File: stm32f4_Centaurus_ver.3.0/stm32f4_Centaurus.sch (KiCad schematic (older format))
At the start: 226 parts, among them IC1 PIC24FJ64GB004, J1 SERIAL1, J2 EXTERNAL_~RST, P1 PICKit3, P10 XA2_12V, P11 CAN0, P12 CAN1, P13 CAN0, P14 CAN1, P15 SERIAL2, P16 SERIAL0, P17 XA2_5V, P18 SWD, P2 SERIAL5_SBDBT, P23 A/D, P24 PWM, P25 A/D_batt, P26 PWM_batt, P27 EMERGENCY_CHECK, P28 I/O_5V, P29 I/O_Variable, P3 ENC0, P30 I/O_5V_batt, P31 I/O_Variable, P4 ENC2, P5 SPI0, P6 ENC3, P7 ENC1, P8 SERIAL4, P9 SERIAL3, Q1 FET_P, Q2 FET_P, Q3 FET_P, Q4 NPN, Q5 NPN, Q6 FET_P, Q7 FET_N, Q8 FET_N, SW1 Main_POWER, SW2 SW1, SW3 SW0, SW4 SW2, SW5 SW3, U1 STM32F407VG, U10 LOGO, U11 CPC1106N, U13 LOGO, U2 AZ1086H, U3 MCP2221A, U4 BD9G101G, U5 MAX3051, U6 MAX3051, U7 AQM1602_BL, U8 OSTBABS4C2B, U9 LOGO, X1 8MHz

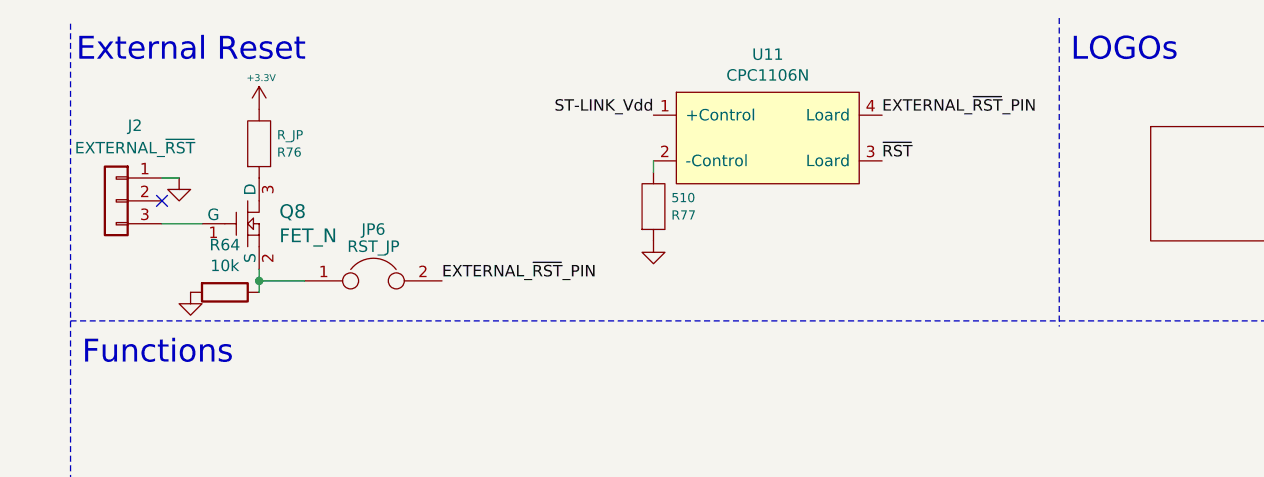
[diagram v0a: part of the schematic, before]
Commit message: 卍配　置　完　了卍
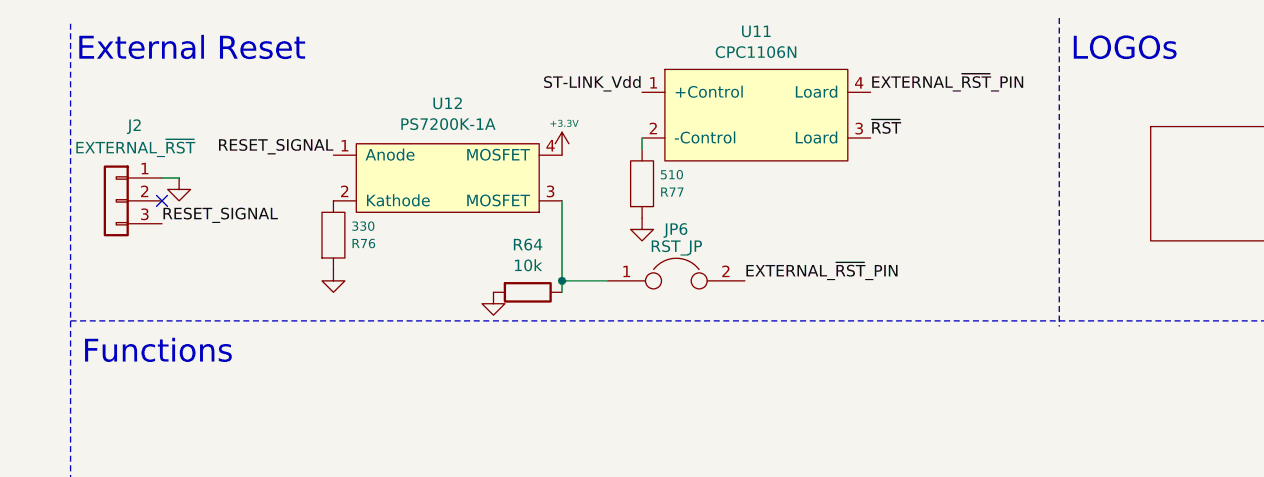
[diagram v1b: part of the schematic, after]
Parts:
- removed Q8: FET_N, Mizz_lib:SOT-23, symbol stm32f4_Centaurus-rescue:MOSFET_N_123-Hori_lib
- added U12: PS7200K-1A, Package_SO:SOP-4_3.8x4.1mm_P2.54mm, symbol Miz:PS7200K-1A
- R76: value R_JP -> 330
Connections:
- net +3V3: now also U12.4 (MOSFET); no longer R76.2
- net GND: now also R76.1
- net RESET_SIGNAL: now reaches J2.3 (Pin_3)
- net RESET_SIGNAL: now also U12.1 (Anode)
- net at JP6.1, R64.1: now also U12.3 (MOSFET)
- new net: R76.2, U12.2 (Kathode)
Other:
- moved on the sheet: JP6, R64, R77, U11
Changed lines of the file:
@@
 L stm32f4_Centaurus-rescue:GND-power #PWR0124
 U 1 1 5E845FAB
-P 17325 1425
-F 0 "#PWR0124" H 17325 1425 30  0001 C CNN
-F 1 "GND" H 17325 1355 30  0001 C CNN
-F 2 "" H 17325 1425 60  0000 C CNN
-F 3 "" H 17325 1425 60  0000 C CNN
-	1    17325 1425
+P 17275 1325
+F 0 "#PWR0124" H 17275 1325 30  0001 C CNN
+F 1 "GND" H 17275 1255 30  0001 C CNN
+F 2 "" H 17275 1325 60  0000 C CNN
+F 3 "" H 17275 1325 60  0000 C CNN
+	1    17275 1325
 	1    0    0    -1
 $EndComp
@@
 Text Label 2225 6825 0    50   ~ 0
 ~RST
-Text Label 18325 1075 0    50   ~ 0
+Text Label 18275 975  0    50   ~ 0
 ~RST
 $Comp
@@
 	1975 5900 2000 5900
 Connection ~ 1975 5900
-Text Label 17325 875  2    50   ~ 0
+Text Label 17275 775  2    50   ~ 0
 ST-LINK_Vdd
 $Comp
 L Miz:CPC1106N U11
 U 1 1 5E762683
-P 17825 975
-F 0 "U11" H 17825 1340 50  0000 C CNN
-F 1 "CPC1106N" H 17825 1249 50  0000 C CNN
-F 2 "Package_SO:SOP-4_3.8x4.1mm_P2.54mm" H 17825 1225 50  0001 C CNN
-F 3 "" H 17825 1225 50  0001 C CNN
-	1    17825 975
+P 17775 875
+F 0 "U11" H 17775 1240 50  0000 C CNN
+F 1 "CPC1106N" H 17775 1149 50  0000 C CNN
+F 2 "Package_SO:SOP-4_3.8x4.1mm_P2.54mm" H 17775 1125 50  0001 C CNN
+F 3 "" H 17775 1125 50  0001 C CNN
+	1    17775 875
 	1    0    0    -1
 $EndComp
@@
 L stm32f4_Centaurus-rescue:R-device R77
 U 1 1 5E7A7A85
-P 17325 1275
-F 0 "R77" H 17403 1313 40  0000 L CNN
-F 1 "510" H 17403 1237 40  0000 L CNN
-F 2 "Mizz_lib:1608_WP" V 17255 1275 30  0001 C CNN
-F 3 "" H 17325 1275 30  0000 C CNN
-	1    17325 1275
+P 17275 1175
+F 0 "R77" H 17353 1213 40  0000 L CNN
+F 1 "510" H 17353 1137 40  0000 L CNN
+F 2 "Mizz_lib:1608_WP" V 17205 1175 30  0001 C CNN
+F 3 "" H 17275 1175 30  0000 C CNN
+	1    17275 1175
 	1    0    0    1
 $EndComp
 Wire Wire Line
-	17325 1075 17325 1125
+	17275 975  17275 1025
 $Comp
 L stm32f4_Centaurus-rescue:+3.3V-power #PWR0139
 U 1 1 5E766875
-P 15600 850
-F 0 "#PWR0139" H 15600 810 30  0001 C CNN
-F 1 "+3.3V" H 15609 988 30  0000 C CNN
-F 2 "" H 15600 850 60  0000 C CNN
-F 3 "" H 15600 850 60  0000 C CNN
-	1    15600 850
-	1    0    0    -1
-$EndComp
-$Comp
-L stm32f4_Centaurus-rescue:MOSFET_N_123-Hori_lib Q8
-U 1 1 5E76467F
-P 15500 1350
-F 0 "Q8" H 15688 1403 60  0000 L CNN
-F 1 "FET_N" H 15688 1297 60  0000 L CNN
-F 2 "Mizz_lib:SOT-23" H 15595 1350 60  0001 C CNN
-F 3 "" H 15595 1350 60  0000 C CNN
-	1    15500 1350
+P 16925 1050
+F 0 "#PWR0139" H 16925 1010 30  0001 C CNN
+F 1 "+3.3V" H 16934 1188 30  0000 C CNN
+F 2 "" H 16925 1050 60  0000 C CNN
+F 3 "" H 16925 1050 60  0000 C CNN
+	1    16925 1050
 	1    0    0    -1
 $EndComp
@@
 L stm32f4_Centaurus-rescue:GND-power #PWR0125
 U 1 1 5F1B4099
-P 15300 1650
-F 0 "#PWR0125" H 15300 1650 30  0001 C CNN
-F 1 "GND" H 15300 1580 30  0001 C CNN
-F 2 "" H 15300 1650 60  0000 C CNN
-F 3 "" H 15300 1650 60  0000 C CNN
-	1    15300 1650
-	1    0    0    -1
-$EndComp
-Wire Wire Line
-	15350 1350 15175 1350
-$Comp
-L stm32f4_Centaurus-rescue:R-device R76
-U 1 1 5F0AF5B9
-P 15600 1000
-F 0 "R76" H 15678 1038 40  0000 L CNN
-F 1 "R_JP" H 15678 962 40  0000 L CNN
-F 2 "Mizz_lib:1608_WP" V 15530 1000 30  0001 C CNN
-F 3 "" H 15600 1000 30  0000 C CNN
-	1    15600 1000
-	1    0    0    1
+P 16625 1650
+F 0 "#PWR0125" H 16625 1650 30  0001 C CNN
+F 1 "GND" H 16625 1580 30  0001 C CNN
+F 2 "" H 16625 1650 60  0000 C CNN
+F 3 "" H 16625 1650 60  0000 C CNN
+	1    16625 1650
+	1    0    0    -1
 $EndComp
 $Comp
 L Device:Jumper JP6
 U 1 1 5EC84997
-P 16100 1600
-F 0 "JP6" H 16100 1825 50  0000 C CNN
-F 1 "RST_JP" H 16100 1750 50  0000 C CNN
-F 2 "Connector_PinHeader_2.54mm:PinHeader_1x02_P2.54mm_Vertical" H 16100 1600 50  0001 C CNN
-F 3 "~" H 16100 1600 50  0001 C CNN
-	1    16100 1600
+P 17425 1600
+F 0 "JP6" H 17425 1825 50  0000 C CNN
+F 1 "RST_JP" H 17425 1750 50  0000 C CNN
+F 2 "Connector_PinHeader_2.54mm:PinHeader_1x02_P2.54mm_Vertical" H 17425 1600 50  0001 C CNN
+F 3 "~" H 17425 1600 50  0001 C CNN
+	1    17425 1600
 	1    0    0    -1
 $EndComp
@@
 Text Notes 14800 650  0    100  ~ 0
 External Reset
-Text Label 16400 1600 0    50   ~ 0
+Text Label 17725 1600 0    50   ~ 0
 EXTERNAL_~RST~_PIN
-Text Label 18325 875  0    50   ~ 0
+Text Label 18275 775  0    50   ~ 0
 EXTERNAL_~RST~_PIN
 $Comp
 L Device:R R64
 U 1 1 5EA261A9
-P 15450 1650
-F 0 "R64" V 15243 1650 50  0000 C CNN
-F 1 "10k" V 15334 1650 50  0000 C CNN
-F 2 "Mizz_lib:1608_WP" V 15380 1650 50  0001 C CNN
-F 3 "~" H 15450 1650 50  0001 C CNN
-	1    15450 1650
-	0    1    1    0
-$EndComp
-Wire Wire Line
-	15800 1600 15600 1600
-Wire Wire Line
-	15600 1600 15600 1550
-Wire Wire Line
-	15600 1600 15600 1650
-Connection ~ 15600 1600
+P 16775 1650
+F 0 "R64" V 16568 1650 50  0000 C CNN
+F 1 "10k" V 16659 1650 50  0000 C CNN
+F 2 "Mizz_lib:1608_WP" V 16705 1650 50  0001 C CNN
+F 3 "~" H 16775 1650 50  0001 C CNN
+	1    16775 1650
+	0    1    1    0
+$EndComp
+Wire Wire Line
+	17125 1600 16925 1600
+Wire Wire Line
+	16925 1600 16925 1650
+Connection ~ 16925 1600
 $Comp
 L Device:R R78
@@
 	21325 3300 21350 3300
 $Comp
-L stm32f4_Centaurus-rescue:+12V-power #PWR?
+L stm32f4_Centaurus-rescue:+12V-power #PWR0140
 U 1 1 5EDC0771
 P 21350 3300
-F 0 "#PWR?" H 21350 3250 20  0001 C CNN
+F 0 "#PWR0140" H 21350 3250 20  0001 C CNN
 F 1 "+12V" H 21350 3438 30  0000 C CNN
 F 2 "" H 21350 3300 60  0000 C CNN
@@
 Wire Wire Line
 	21350 3300 21375 3300
+$Comp
+L Miz:PS7200K-1A U12
+U 1 1 5E8C834E
+P 16425 1150
+F 0 "U12" H 16425 1475 50  0000 C CNN
+F 1 "PS7200K-1A" H 16425 1384 50  0000 C CNN
+F 2 "Package_SO:SOP-4_3.8x4.1mm_P2.54mm" H 16425 1150 50  0001 C CNN
+F 3 "" H 16425 1150 50  0001 C CNN
+	1    16425 1150
+	1    0    0    -1
+$EndComp
+Text Label 15175 1350 0    50   ~ 0
+RESET_SIGNAL
+Text Label 15925 1050 2    50   ~ 0
+RESET_SIGNAL
+Wire Wire Line
+	16925 1250 16925 1600
+$Comp
+L stm32f4_Centaurus-rescue:R-device R76
+U 1 1 5EA4ACF2
+P 15925 1400
+F 0 "R76" H 16003 1438 40  0000 L CNN
+F 1 "330" H 16003 1362 40  0000 L CNN
+F 2 "Mizz_lib:1608_WP" V 15855 1400 30  0001 C CNN
+F 3 "" H 15925 1400 30  0000 C CNN
+	1    15925 1400
+	1    0    0    1
+$EndComp
+$Comp
+L stm32f4_Centaurus-rescue:GND-power #PWR0172
+U 1 1 5EA4B42A
+P 15925 1550
+F 0 "#PWR0172" H 15925 1550 30  0001 C CNN
+F 1 "GND" H 15925 1480 30  0001 C CNN
+F 2 "" H 15925 1550 60  0000 C CNN
+F 3 "" H 15925 1550 60  0000 C CNN
+	1    15925 1550
+	1    0    0    -1
+$EndComp
 $EndSCHEMATC
